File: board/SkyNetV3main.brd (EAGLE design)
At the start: 160 x 100 mm, 67 parts, among them IC1 HC_05, IC2 RF4463PRO, IC3 LPC1768, IC4 BCX17, IC5 TPS63001, IC6 MCP73871-2CCI/ML, Q1 32.768KHz, Q2 12MHz, Q3 IRLM6402, Q4 BSS138, X1 BAT

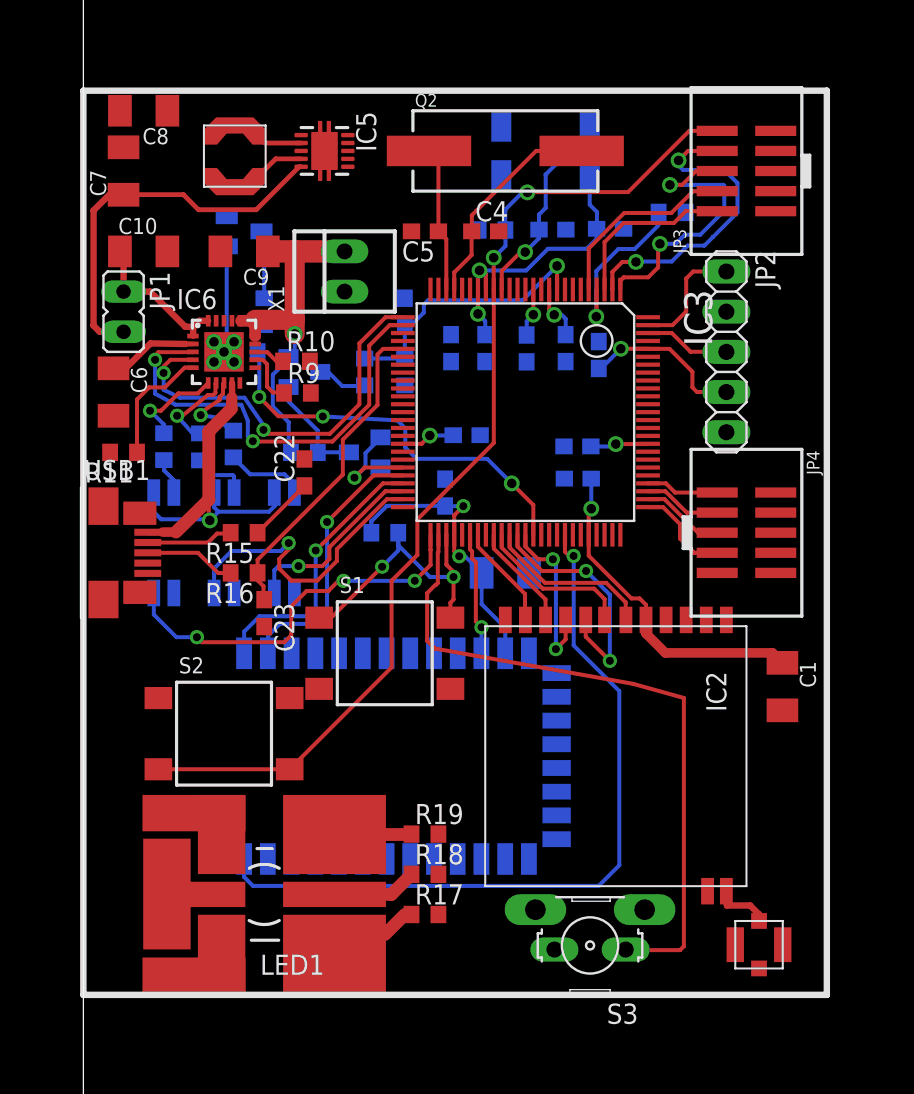
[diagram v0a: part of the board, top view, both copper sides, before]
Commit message: board further
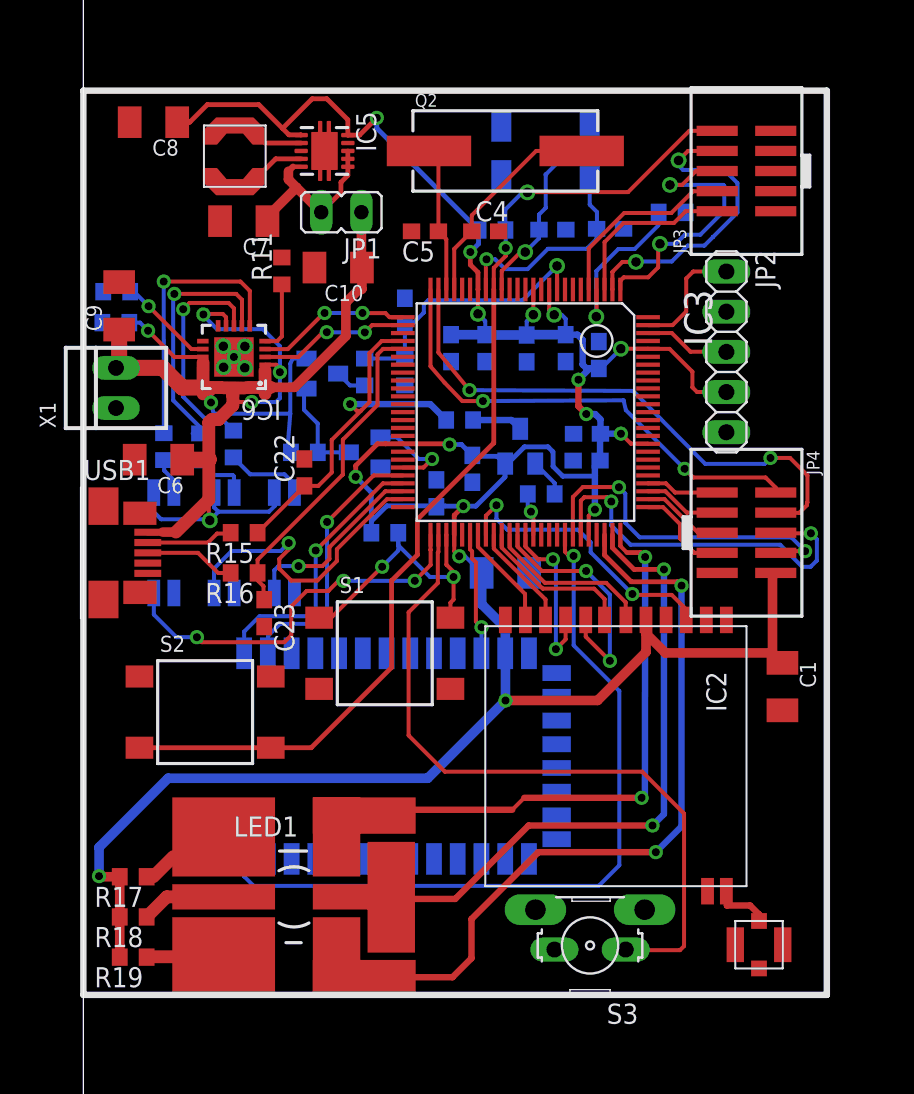
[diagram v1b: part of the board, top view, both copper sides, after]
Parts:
- moved IC4 22.1 mm to (27.6, 46.1), turned to 0 degrees
- moved R3 20.8 mm to (28.9, 43.1), turned to 180 degrees
- moved R19 20.0 mm to (3.15, 13.8), turned to 180 degrees
- moved R18 18.6 mm to (3.15, 16.4), turned to 180 degrees
- moved R17 18.6 mm to (3.15, 18.9), turned to 180 degrees
- moved X1 16.2 mm to (2.06, 49.8)
- moved R11 15.2 mm to (12.5, 57.2), turned to 90 degrees
- moved JP1 15.1 mm to (16.3, 60.9), turned to 90 degrees
- moved R4 14.1 mm to (23.8, 47.8), turned to 180 degrees
- moved R9 13.1 mm to (2.11, 55.9), flipped to the bottom
- moved C10 12.3 mm to (16.1, 57.4), turned to 180 degrees
- moved R10 11.7 mm to (2.05, 53.9), flipped to the bottom
- moved C9 8.61 mm to (2.26, 55.0), turned to 90 degrees
- moved C7 8.23 mm to (10.1, 60.3), turned to 180 degrees
- moved C6 5.13 mm to (4.74, 45.3), turned to 180 degrees
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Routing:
- net +3V3: track 66.4 -> 193.3 mm, vias 9 -> 16
- net LED_B: track 0.00 -> 50.0 mm, vias 0 -> 2
- net LED_G: track 0.00 -> 42.1 mm, vias 0 -> 2
- net LED_R: track 0.00 -> 38.9 mm, vias 0 -> 2
- net SCL_EXT: track 0.00 -> 35.0 mm, vias 0 -> 2
- net SDA_EXT: track 0.00 -> 30.5 mm, vias 0 -> 2
- net EXT_GPIO0: track 0.00 -> 24.1 mm, vias 0 -> 2
- net USB-CON: track 25.5 -> 2.73 mm, vias 3 -> 1
- net EXT_GPIO1: track 0.00 -> 22.0 mm, vias 0 -> 2
- net USB-D+: track 4.19 -> 24.6 mm, vias 0 -> 1
- net RF-GPIO0: track 0.00 -> 18.4 mm, vias 0 -> 2
- net CHGSEL_H: track 27.8 -> 9.55 mm
- net CHGSEL_L: track 25.3 -> 9.77 mm
- net +5V: track 31.6 -> 44.3 mm, vias 1 -> 4
- net VCC: track 24.4 -> 11.8 mm
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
